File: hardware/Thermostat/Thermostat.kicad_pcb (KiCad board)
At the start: 2 copper layers, 106 x 75 mm, 44 parts, among them J1 MainConnectorr, J2 Screw_Terminal_01x02, J3 AVR-ISP-6, K1 G6E, K2 G6E, K3 G6E, K4 G6E, SW1_COOL1 Conn_02x03_Top_Bottom, SW1_FAN1 Conn_02x03_Top_Bottom, SW1_UP1 SW_Push, SW2_DOWN1 SW_Push, SW5_RESET1 SW_Push, U2 NCP718xSN500, U4 DS3231MZ, U5 ATmega88-20A, U6 TMP116xxDRV, U7 THVD1500, Y1 Crystal

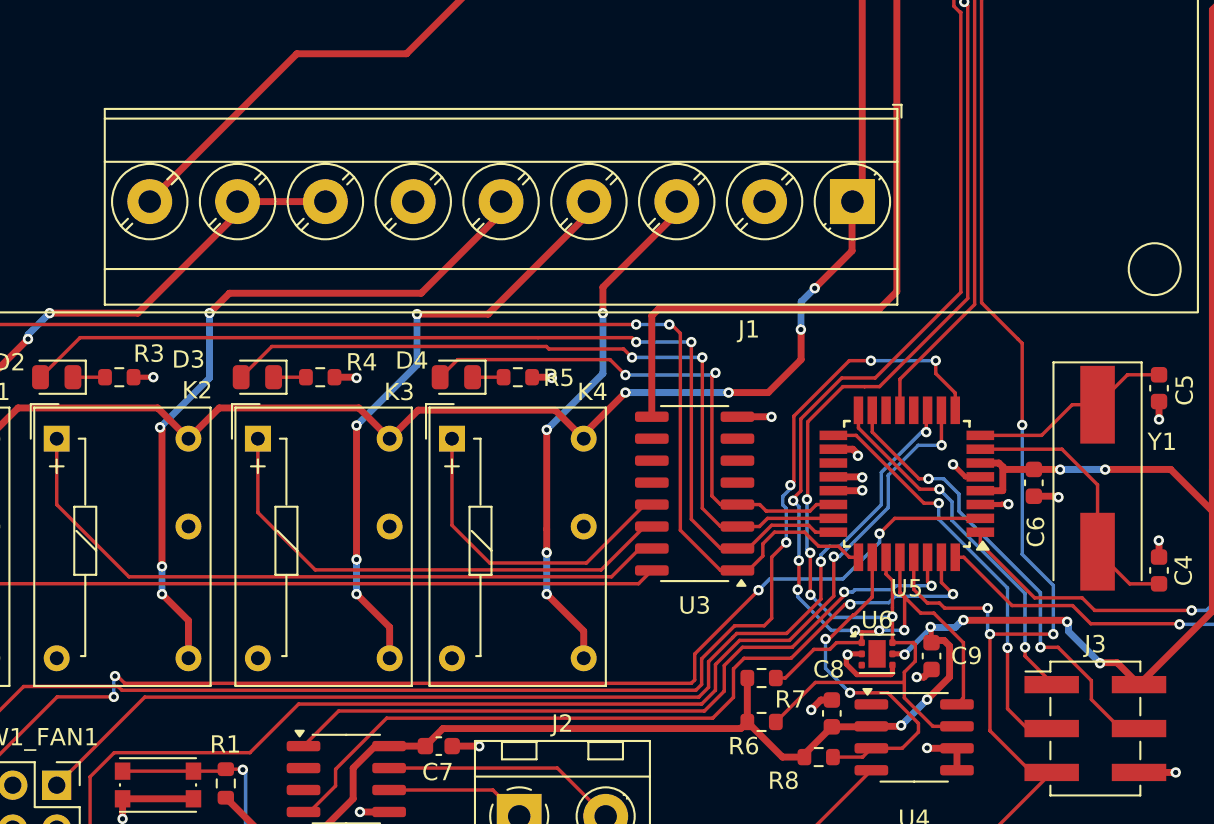
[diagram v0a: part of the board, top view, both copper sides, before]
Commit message: Tweaks?
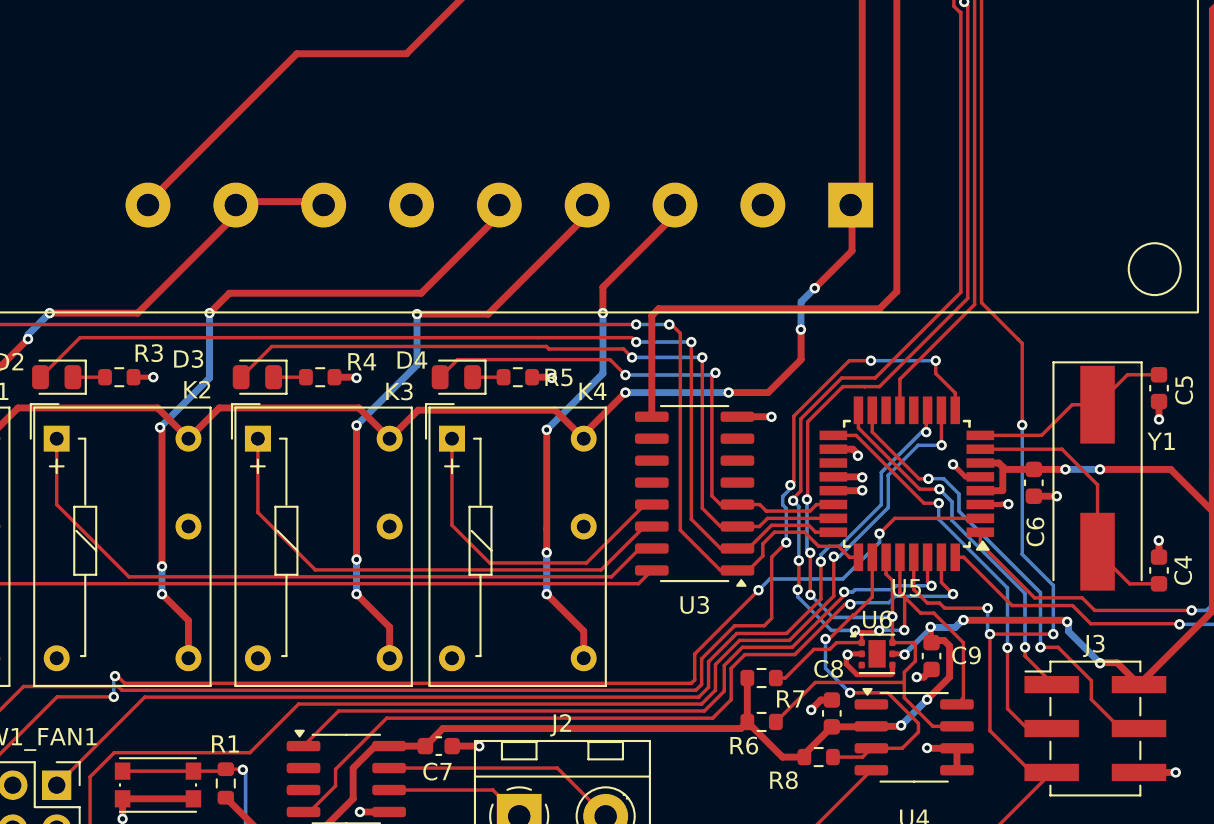
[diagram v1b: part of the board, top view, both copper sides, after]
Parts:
- J1: moved to B.Cu
- moved J1 0.22 mm to (183.1, 82.5)
